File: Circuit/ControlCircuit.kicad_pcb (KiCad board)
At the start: 2 copper layers, 79 parts, among them CON501 AVR-ISP-10, IC501 ATMEGA644-A, K201 Meisei-m4-24h, K202 Meisei-m4-24h, K203 Meisei-m4-24h, K204 Meisei-m4-24h, K205 Meisei-m4-24h, K206 Meisei-m4-24h, K207 Meisei-m4-24h, K208 Meisei-m4-24h, P101 CONN_01X08, P102 CONN_01X08, P103 CONN_01X08, P104 CONN_01X08, P105 CONN_01X08, P106 CONN_01X08, P107 CONN_01X02, Q201 Q_NPN_BCE, Q202 Q_NPN_BCE, Q203 Q_NPN_BCE, Q204 Q_NPN_BCE, Q205 Q_NPN_BCE, Q206 Q_NPN_BCE, Q207 Q_NPN_BCE, Q208 Q_NPN_BCE, U301 LTV-817, U302 LTV-817, U303 LTV-817, U304 LTV-817, U305 LTV-817, U306 LTV-817, U307 LTV-817, U308 LTV-817, Y501 Crystal

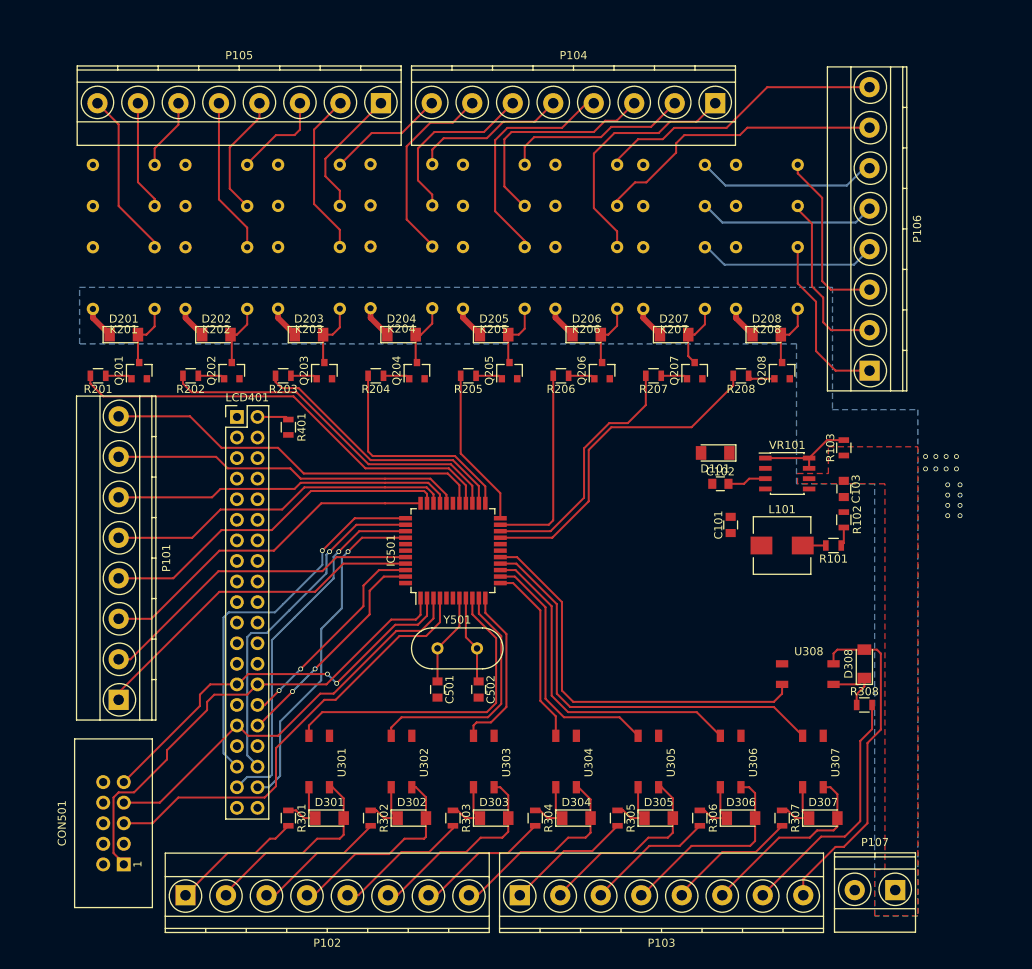
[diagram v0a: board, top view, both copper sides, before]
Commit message: PCB. Pours mostly complete. Almost done?
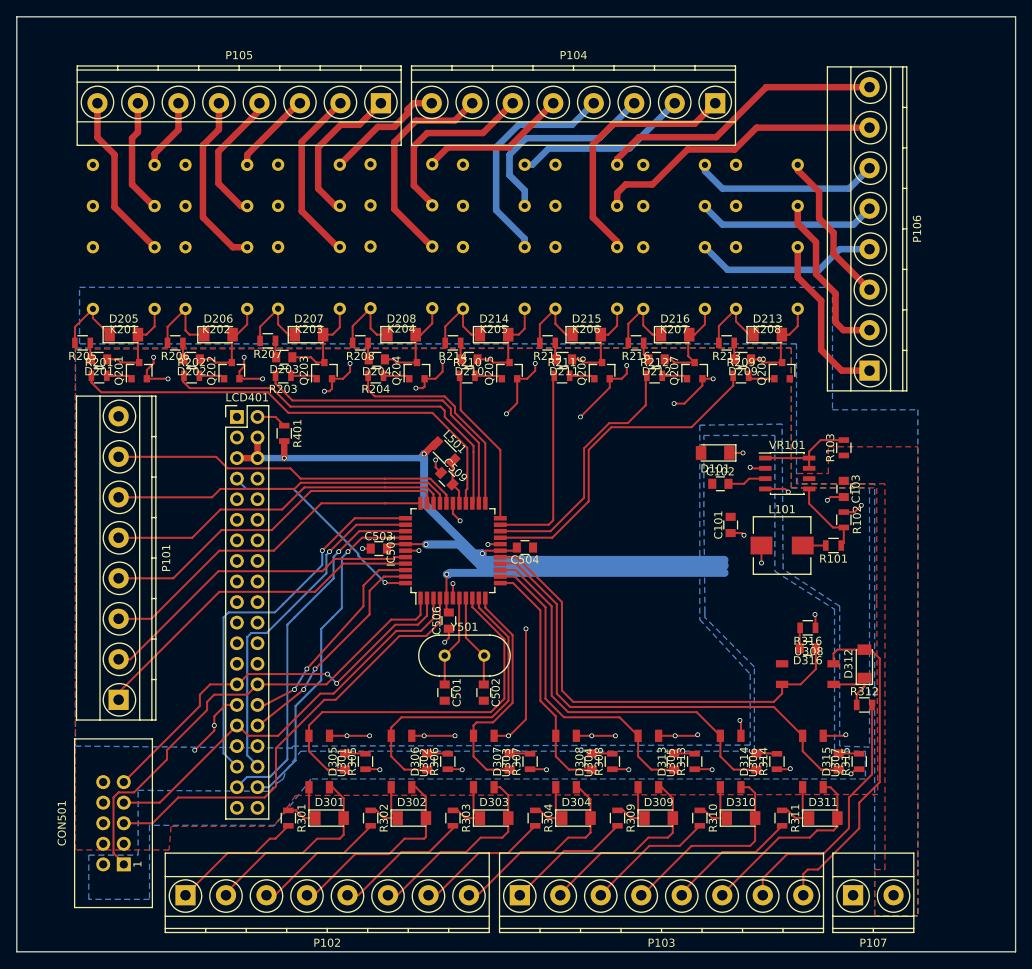
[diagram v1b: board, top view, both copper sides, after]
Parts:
- added C503: 100uF, Capacitors_SMD:C_0805, F.Cu at (92.5, 98.8)
- added C504: 100uF, Capacitors_SMD:C_0805, F.Cu at (110.5, 98.7)
- added C506: 100uF, Capacitors_SMD:C_0805, F.Cu at (101.1, 107.7)
- added C509: 100uF, Capacitors_SMD:C_0805, F.Cu at (100.8, 90.2)
- added D209: LED, Capacitors_SMD:C_0805, F.Cu at (137.4, 75.4)
- added D210: LED, Capacitors_SMD:C_0805, F.Cu at (103.6, 75.4)
- added D211: LED, Capacitors_SMD:C_0805, F.Cu at (115.3, 75.4)
- added D212: LED, Capacitors_SMD:C_0805, F.Cu at (126.7, 75.4)
- added D213: D, Diodes_SMD:D_MiniMELF_Standard, F.Cu at (140.5, 72.4)
- added D214: D, Diodes_SMD:D_MiniMELF_Standard, F.Cu at (106.7, 72.4)
- added D215: D, Diodes_SMD:D_MiniMELF_Standard, F.Cu at (118.1, 72.4)
- added D216: D, Diodes_SMD:D_MiniMELF_Standard, F.Cu at (129.0, 72.4)
- added D309: D, Diodes_SMD:D_MiniMELF_Standard, F.Cu at (127.0, 132.1)
- added D310: D, Diodes_SMD:D_MiniMELF_Standard, F.Cu at (137.2, 132.1)
- added D311: D, Diodes_SMD:D_MiniMELF_Standard, F.Cu at (147.3, 132.1)
- added D312: D, Diodes_SMD:D_MiniMELF_Standard, F.Cu at (152.4, 113.0)
- added D313: LED, Capacitors_SMD:C_0805, F.Cu at (128.9, 125.1)
- added D314: LED, Capacitors_SMD:C_0805, F.Cu at (139.1, 125.1)
- added D315: LED, Capacitors_SMD:C_0805, F.Cu at (149.2, 125.1)
- added D316: LED, Capacitors_SMD:C_0805, F.Cu at (145.4, 111.1)
- added L501: 10uH, Capacitors_SMD:C_1206, F.Cu at (100.6, 86.9)
- added R209: 10kR, Resistors_SMD:R_0805, F.Cu at (137.2, 77.5)
- added R210: 10kR, Resistors_SMD:R_0805, F.Cu at (103.4, 77.5)
- added R211: 10kR, Resistors_SMD:R_0805, F.Cu at (115.1, 77.5)
- added R212: 10kR, Resistors_SMD:R_0805, F.Cu at (126.5, 77.5)
- added R213: 10kR, Resistors_SMD:R_0805, F.Cu at (135.4, 73.4)
- added R214: 10kR, Resistors_SMD:R_0805, F.Cu at (101.6, 73.4)
- added R215: 10kR, Resistors_SMD:R_0805, F.Cu at (113.3, 73.4)
- added R216: 10kR, Resistors_SMD:R_0805, F.Cu at (124.2, 73.4)
- added R309: 2kR, Resistors_SMD:R_0805, F.Cu at (121.9, 132.1)
- added R310: 2kR, Resistors_SMD:R_0805, F.Cu at (132.1, 132.1)
- added R311: 2kR, Resistors_SMD:R_0805, F.Cu at (142.2, 132.1)
- added R312: 2kR, Resistors_SMD:R_0805, F.Cu at (152.4, 118.1)
- added R313: 1kR, Resistors_SMD:R_0805, F.Cu at (131.4, 125.1)
- added R314: 1kR, Resistors_SMD:R_0805, F.Cu at (141.6, 125.1)
- added R315: 1kR, Resistors_SMD:R_0805, F.Cu at (151.8, 125.1)
- added R316: 1kR, Resistors_SMD:R_0805, F.Cu at (145.4, 108.6)
- D201, D202, D203, D204, D305, D306, D307, D308: value D -> LED; footprint Diodes_SMD:D_MiniMELF_Standard -> Capacitors_SMD:C_0805
- R305, R306, R307, R308: value 2kR -> 1kR
- moved R207 47.8 mm to (78.7, 73.2)
- moved R206 47.8 mm to (67.3, 73.4)
- moved R205 47.8 mm to (55.9, 73.4)
- moved R208 47.2 mm to (90.2, 73.4)
- moved D205 45.7 mm to (61.0, 72.4)
- moved D206 45.5 mm to (72.6, 72.4)
- moved D207 45.1 mm to (83.8, 72.4)
- moved D208 45.1 mm to (95.2, 72.4)
- moved D305 39.4 mm to (88.3, 125.1), turned to 90 degrees
- moved D306 39.4 mm to (98.4, 125.1), turned to 90 degrees
- moved D307 39.4 mm to (108.6, 125.1), turned to 90 degrees
- moved D308 35.8 mm to (118.7, 125.1)
- moved R306 31.9 mm to (101.0, 125.1), turned to 90 degrees
- moved R307 31.9 mm to (111.1, 125.1), turned to 90 degrees
- moved R308 31.9 mm to (121.3, 125.1), turned to 90 degrees
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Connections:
- D201 pad 1: +24V -> Net-(D201-Pad1)
- D202 pad 1: +24V -> Net-(D202-Pad1)
- D203 pad 1: +24V -> Net-(D203-Pad1)
- D204 pad 1: +24V -> Net-(D204-Pad1)
- D205 pad 2: Net-(D205-Pad2) -> Net-(D201-Pad1)
- D206 pad 2: Net-(D206-Pad2) -> Net-(D202-Pad1)
- D207 pad 2: Net-(D207-Pad2) -> Net-(D203-Pad1)
- D208 pad 2: Net-(D208-Pad2) -> Net-(D204-Pad1)
- D305 pad 1: Net-(D305-Pad1) -> /RelayInputs/I1
- D305 pad 2: /RelayInputs/RI5K -> Net-(D305-Pad2)
- D306 pad 1: Net-(D306-Pad1) -> /RelayInputs/I2
- D306 pad 2: /RelayInputs/RI6K -> Net-(D306-Pad2)
- D307 pad 1: Net-(D307-Pad1) -> /RelayInputs/I3
- D307 pad 2: /RelayInputs/RI7K -> Net-(D307-Pad2)
- D308 pad 1: Net-(D308-Pad1) -> /RelayInputs/I4
- D308 pad 2: /RelayInputs/RI8K -> Net-(D308-Pad2)
- IC501 pad 27: /AVCC -> Net-(C509-Pad2)
- K201 pad 1: Net-(D201-Pad2) -> Net-(D201-Pad1)
- K202 pad 1: Net-(D202-Pad2) -> Net-(D202-Pad1)
- K203 pad 1: Net-(D203-Pad2) -> Net-(D203-Pad1)
- K204 pad 1: Net-(D204-Pad2) -> Net-(D204-Pad1)
- K205 pad 1: Net-(D205-Pad2) -> Net-(D210-Pad1)
- K206 pad 1: Net-(D206-Pad2) -> Net-(D211-Pad1)
- K207 pad 1: Net-(D207-Pad2) -> Net-(D212-Pad1)
- K208 pad 1: Net-(D208-Pad2) -> Net-(D209-Pad1)
- P107 pad 1: +24V -> GND
- P107 pad 2: GND -> +24V
- Q201 pad 1: GNDREF -> GND
- Q201 pad 2: Net-(D201-Pad2) -> Net-(D201-Pad1)
- Q202 pad 1: GNDREF -> GND
- Q202 pad 2: Net-(D202-Pad2) -> Net-(D202-Pad1)
- Q203 pad 1: GNDREF -> GND
- Q203 pad 2: Net-(D203-Pad2) -> Net-(D203-Pad1)
- Q204 pad 1: GNDREF -> GND
- Q204 pad 2: Net-(D204-Pad2) -> Net-(D204-Pad1)
- Q205 pad 1: GNDREF -> GND
- Q205 pad 2: Net-(D205-Pad2) -> Net-(D210-Pad1)
- Q206 pad 1: GNDREF -> GND
- Q206 pad 2: Net-(D206-Pad2) -> Net-(D211-Pad1)
- Q207 pad 1: GNDREF -> GND
- Q207 pad 2: Net-(D207-Pad2) -> Net-(D212-Pad1)
- Q208 pad 1: GNDREF -> GND
- Q208 pad 2: Net-(D208-Pad2) -> Net-(D209-Pad1)
- R201 pad 1: Net-(Q201-Pad3) -> /RelayOutputs/O1
- R201 pad 2: /RelayOutputs/O1 -> Net-(Q201-Pad3)
- R202 pad 1: Net-(Q202-Pad3) -> /RelayOutputs/O2
- R202 pad 2: /RelayOutputs/O2 -> Net-(Q202-Pad3)
- R205 pad 1: Net-(Q205-Pad3) -> Net-(D201-Pad2)
- R205 pad 2: /RelayOutputs/O5 -> +24V
- R206 pad 1: Net-(Q206-Pad3) -> Net-(D202-Pad2)
- R206 pad 2: /RelayOutputs/O6 -> +24V
- R207 pad 1: Net-(Q207-Pad3) -> Net-(D203-Pad2)
- R207 pad 2: /RelayOutputs/O7 -> +24V
- R208 pad 1: Net-(Q208-Pad3) -> Net-(D204-Pad2)
- R208 pad 2: /RelayOutputs/O8 -> +24V
- R305 pad 1: Net-(D305-Pad1) -> +3V3
- R305 pad 2: /RelayInputs/RI5A -> Net-(D305-Pad2)
- R306 pad 1: Net-(D306-Pad1) -> +3V3
- R306 pad 2: /RelayInputs/RI6A -> Net-(D306-Pad2)
- R307 pad 1: Net-(D307-Pad1) -> +3V3
- R307 pad 2: /RelayInputs/RI7A -> Net-(D307-Pad2)
- R308 pad 1: Net-(D308-Pad1) -> +3V3
- R308 pad 2: /RelayInputs/RI8A -> Net-(D308-Pad2)
- U305 pad 1: Net-(D305-Pad1) -> Net-(D309-Pad1)
- U306 pad 1: Net-(D306-Pad1) -> Net-(D310-Pad1)
- U307 pad 1: Net-(D307-Pad1) -> Net-(D311-Pad1)
- U308 pad 1: Net-(D308-Pad1) -> Net-(D312-Pad1)
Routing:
- net +3V3: track 0.00 -> 185.4 mm, vias 0 -> 17
- net GND: track 0.00 -> 117.2 mm, vias 0 -> 38
- net /AVCC: track 47.8 -> 0.00 mm
- net +24V: track 32.4 -> 77.4 mm
- net /LCDTouchScreen/RST: track 0.00 -> 26.4 mm, vias 0 -> 1
- net Net-(D203-Pad1): track 0.00 -> 12.5 mm
- net Net-(D210-Pad1): track 0.00 -> 12.4 mm
- net Net-(D201-Pad1): track 0.00 -> 12.3 mm
- net Net-(D209-Pad1): track 0.00 -> 12.2 mm
- net Net-(D212-Pad1): track 0.00 -> 12.1 mm
- net Net-(D204-Pad1): track 0.00 -> 12.1 mm
- net Net-(D202-Pad1): track 0.00 -> 12.1 mm
- net Net-(D211-Pad1): track 0.00 -> 11.9 mm
- net /RelayInputs/I2: track 30.0 -> 38.7 mm
- net /RelayInputs/I3: track 20.8 -> 29.3 mm
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- added copper zone on B.Cu, net +3V3
- added copper zone on B.Cu, net GND
- added copper zone on F.Cu, net GND
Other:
- board outline added: 123.3 x 115.4 mm

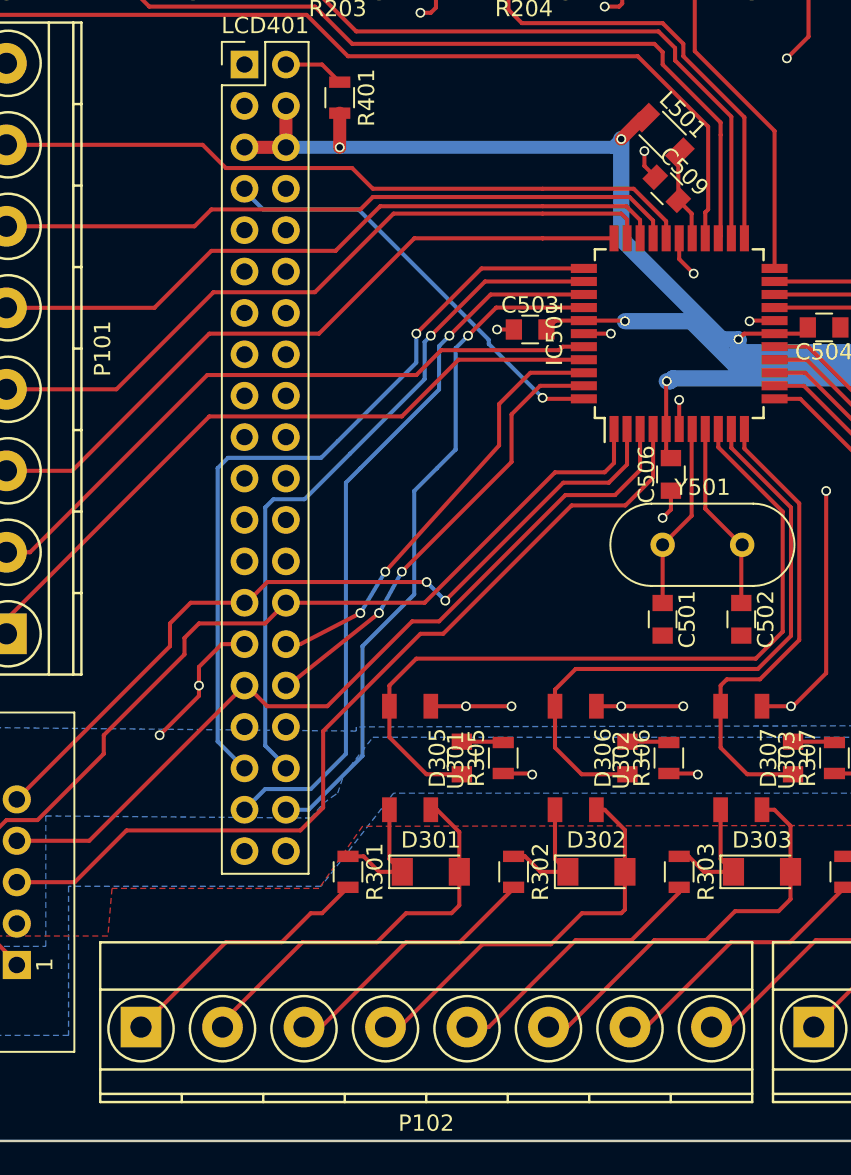
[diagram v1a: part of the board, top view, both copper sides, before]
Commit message: Minor tweak
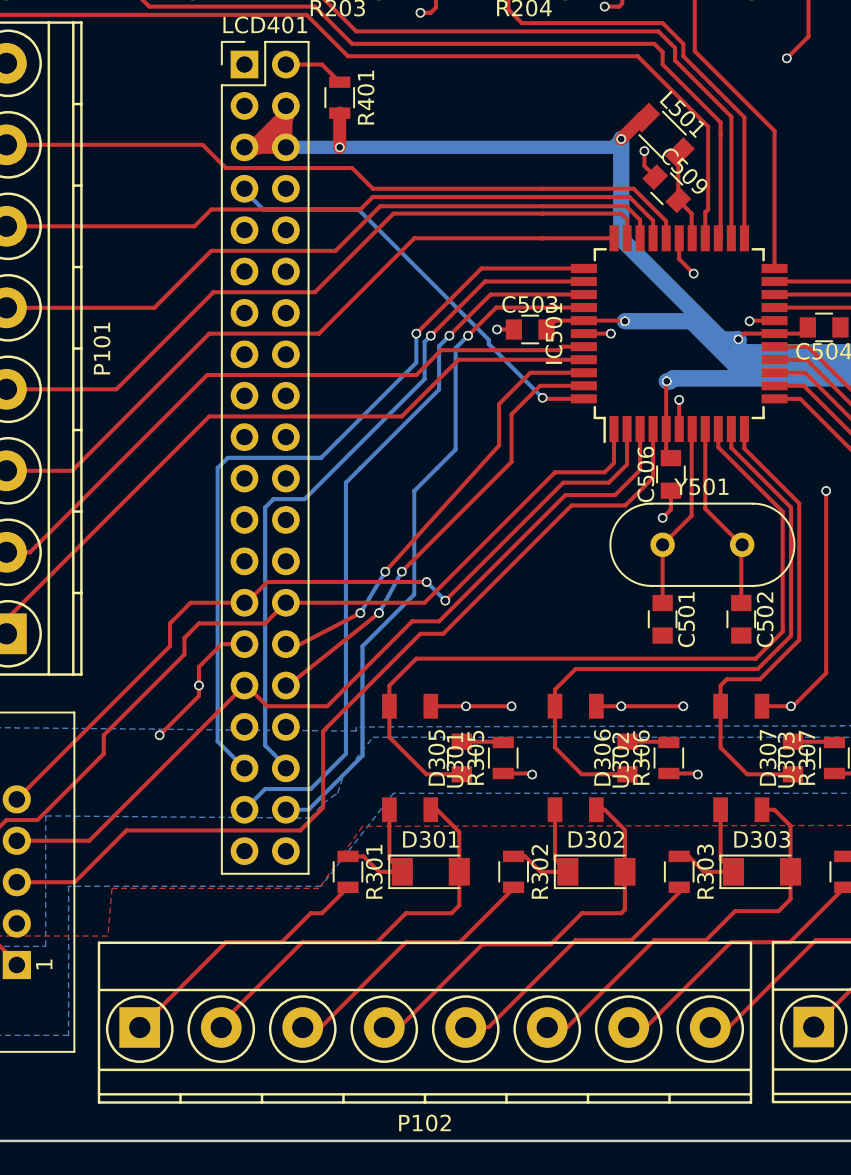
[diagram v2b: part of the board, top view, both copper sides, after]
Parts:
- moved P102 0.08 mm to (68.5, 141.6)
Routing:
- net +3V3: track 185.4 -> 189.4 mm
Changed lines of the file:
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@@
     (thickness 1.6)
     (drawings 12)
-    (tracks 985)
+    (tracks 990)
     (zones 0)
     (modules 116)
@@
   )
   (setup
-    (last_trace_width 0.25)
+    (last_trace_width 1)
     (user_trace_width 0.8)
     (user_trace_width 1)
@@
   )
   (module Connectors_Terminal_Blocks:TerminalBlock_Pheonix_MKDS1.5-8pol (layer F.Cu)
-    (at 68.58 141.605)
+    (at 68.5038 141.6304)
     (descr "8-way 5mm pitch terminal block, Phoenix MKDS series")
     (fp_text reference P102 (at 17.5 5.9) (layer F.SilkS)
@@
   (gr_line (start 47.752 148.59) (end 47.752 33.147) (angle 90) (layer Edge.Cuts) (width 0.15))
   (gr_line (start 68.58 80.01) (end 157.48 80.01) (angle 90) (layer Eco1.User) (width 0.2))
-  (gr_text "Screen circuit board outline" (at 85.09 137.16) (layer Eco1.User)
+  (gr_text "Screen circuit board outline" (at 85.0138 133.3246) (layer Eco1.User)
     (effects (font (size 1.5 1.5) (thickness 0.3)))
   )
@@
   (gr_line (start 68.58 80.01) (end 68.58 93.98) (angle 90) (layer Eco1.User) (width 0.2))
   (gr_line (start 68.58 93.98) (end 68.58 107.95) (angle 90) (layer Eco1.User) (width 0.2))
+  (segment (start 74.93 87.63) (end 75.565 87.63) (width 1) (layer F.Cu) (net 1))
+  (segment (start 75.565 87.63) (end 77.47 85.725) (width 1) (layer F.Cu) (net 1))
+  (segment (start 77.47 85.725) (end 77.47 85.09) (width 1) (layer F.Cu) (net 1))
   (segment (start 105.2322 99.4156) (end 104.2162 99.4156) (width 1) (layer B.Cu) (net 1))
   (segment (start 98.044 93.2434) (end 98.044 87.122) (width 1) (layer B.Cu) (net 1))
@@
   (via (at 102.743 126.111) (size 0.6) (drill 0.4) (layers F.Cu B.Cu) (net 1))
   (segment (start 102.677 126.045) (end 102.743 126.111) (width 0.25) (layer F.Cu) (net 1))
-  (segment (start 77.47 87.63) (end 77.47 85.09) (width 0.8) (layer F.Cu) (net 1))
-  (segment (start 74.93 87.63) (end 77.47 87.63) (width 0.8) (layer F.Cu) (net 1))
+  (segment (start 77.47 87.63) (end 77.47 86.106) (width 0.8) (layer F.Cu) (net 1))
+  (segment (start 77.47 86.106) (end 77.47 85.09) (width 0.8) (layer F.Cu) (net 1))
+  (segment (start 74.93 87.63) (end 75.8444 87.63) (width 0.8) (layer F.Cu) (net 1))
+  (segment (start 75.8444 87.63) (end 77.47 87.63) (width 0.8) (layer F.Cu) (net 1))
   (segment (start 141.605 126.045) (end 143.195 126.045) (width 0.25) (layer F.Cu) (net 1))
   (via (at 143.256 125.984) (size 0.6) (drill 0.4) (layers F.Cu B.Cu) (net 1))
@@
   (segment (start 83.82 128.27) (end 83.82 131.29) (width 0.25) (layer F.Cu) (net 98))
   (segment (start 83.82 131.29) (end 84.61 132.08) (width 0.25) (layer F.Cu) (net 98))
-  (segment (start 73.58 141.605) (end 73.58 141.304) (width 0.25) (layer F.Cu) (net 99))
   (segment (start 73.58 141.304) (end 78.486 136.398) (width 0.25) (layer F.Cu) (net 99))
   (segment (start 78.486 136.398) (end 83.058 136.398) (width 0.25) (layer F.Cu) (net 99))
   (segment (start 83.058 136.398) (end 84.836 134.62) (width 0.25) (layer F.Cu) (net 99))
+  (segment (start 73.58 141.605) (end 73.58 141.304) (width 0.25) (layer F.Cu) (net 99))
   (segment (start 84.836 134.62) (end 87.63 134.62) (width 0.25) (layer F.Cu) (net 99))
   (segment (start 87.63 134.62) (end 88.11 134.14) (width 0.25) (layer F.Cu) (net 99))
@@
   (segment (start 93.091 132.08) (end 94.77 132.08) (width 0.25) (layer F.Cu) (net 100))
   (segment (start 92.141 131.13) (end 93.091 132.08) (width 0.25) (layer F.Cu) (net 100))
-  (segment (start 83.58 141.605) (end 84.455 141.605) (width 0.25) (layer F.Cu) (net 101))
   (segment (start 84.455 141.605) (end 89.535 136.525) (width 0.25) (layer F.Cu) (net 101))
   (segment (start 89.535 136.525) (end 93.726 136.525) (width 0.25) (layer F.Cu) (net 101))
+  (segment (start 83.58 141.605) (end 84.455 141.605) (width 0.25) (layer F.Cu) (net 101))
   (segment (start 93.726 136.525) (end 95.631 134.62) (width 0.25) (layer F.Cu) (net 101))
   (segment (start 95.631 134.62) (end 98.044 134.62) (width 0.25) (layer F.Cu) (net 101))
@@
   (segment (start 89.916 141.605) (end 95.25 136.271) (width 0.25) (layer F.Cu) (net 111))
   (segment (start 101.6 133.35) (end 101.6 133.03) (width 0.25) (layer F.Cu) (net 111))
-  (segment (start 78.58 141.605) (end 79.629 141.605) (width 0.25) (layer F.Cu) (net 112))
   (segment (start 79.629 141.605) (end 84.836 136.398) (width 0.25) (layer F.Cu) (net 112))
   (segment (start 84.836 136.398) (end 88.138 136.398) (width 0.25) (layer F.Cu) (net 112))
   (segment (start 88.138 136.398) (end 91.44 133.096) (width 0.25) (layer F.Cu) (net 112))
+  (segment (start 78.58 141.605) (end 79.629 141.605) (width 0.25) (layer F.Cu) (net 112))
   (segment (start 91.44 133.096) (end 91.44 133.03) (width 0.25) (layer F.Cu) (net 112))
   (segment (start 68.58 141.605) (end 73.787 136.398) (width 0.25) (layer F.Cu) (net 113))
